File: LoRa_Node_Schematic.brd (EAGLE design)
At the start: 51 x 23 mm, 52 parts, among them J1 ZX62D-B-5PA8, J3 B2B-PH-K-S(LF)(SN), U1 ATSAMD21G18A-AU, U2 RFM95W-868S2SMALL, U3 AP2112K-3.3, U4 MCP73831-2ACI/OT, U5 SHT40-AD1B-R2, Y1 32.768KHZ

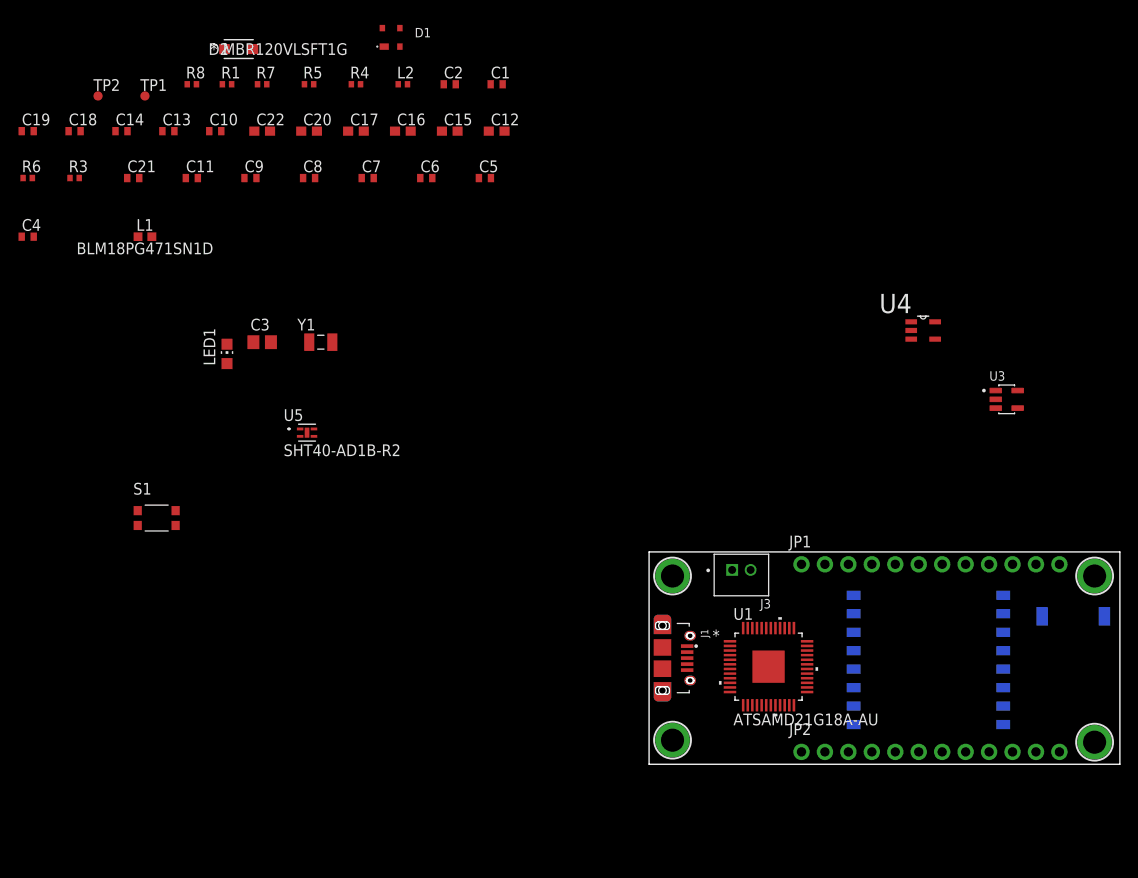
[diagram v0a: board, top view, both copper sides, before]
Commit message: update
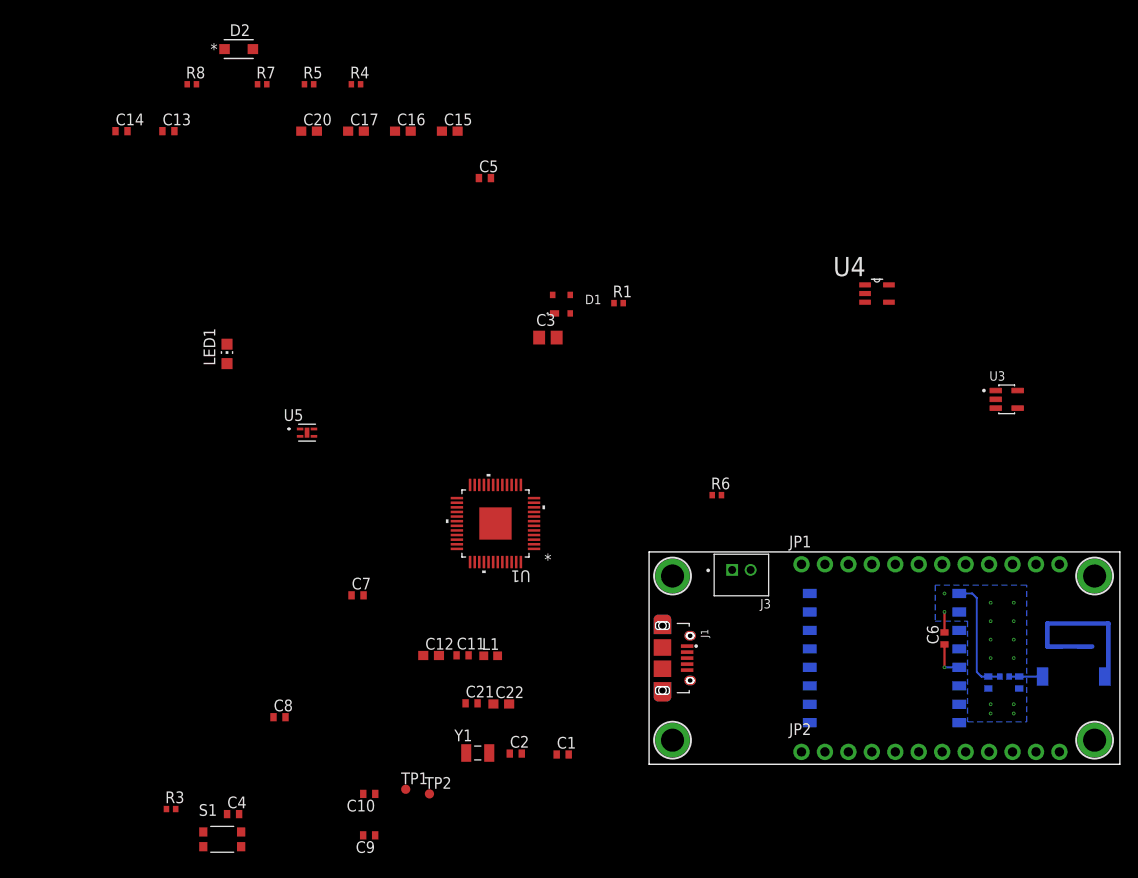
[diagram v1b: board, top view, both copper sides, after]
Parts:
- moved C19 122.9 mm to (40.1, 8.85), flipped to the bottom, turned to 270 degrees
- moved C18 115.6 mm to (36.8, 8.85), flipped to the bottom, turned to 270 degrees
- moved L2 91.5 mm to (38.5, 9.50), flipped to the bottom, turned to 180 degrees
- moved TP2 83.7 mm to (-23.8, -3.21)
- moved R6 82.2 mm to (7.34, 29.1)
- moved TP1 80.2 mm to (-26.4, -2.71)
- moved C6 75.1 mm to (32.0, 13.6), turned to 90 degrees
- moved C10 73.7 mm to (-30.3, -3.21), turned to 180 degrees
- moved C1 73.0 mm to (-9.36, 1.06)
- moved C2 72.9 mm to (-14.4, 1.16)
- moved C9 72.4 mm to (-30.3, -7.70), turned to 180 degrees
- moved R3 69.1 mm to (-51.8, -4.85)
- moved C21 67.7 mm to (-19.2, 6.60)
- moved C22 67.2 mm to (-16.0, 6.53)
- moved C4 66.4 mm to (-45.1, -5.40)
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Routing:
- net ANTENNA: track 0.00 -> 12.8 mm
- net +3V3: track 0.00 -> 4.08 mm, vias 0 -> 1
- net ANTENNA_L: track 0.00 -> 3.88 mm
- net GND: track 0.00 -> 2.22 mm, vias 0 -> 14
- added copper zone on layer 16, net GND
- added copper zone on layer 3, net GND

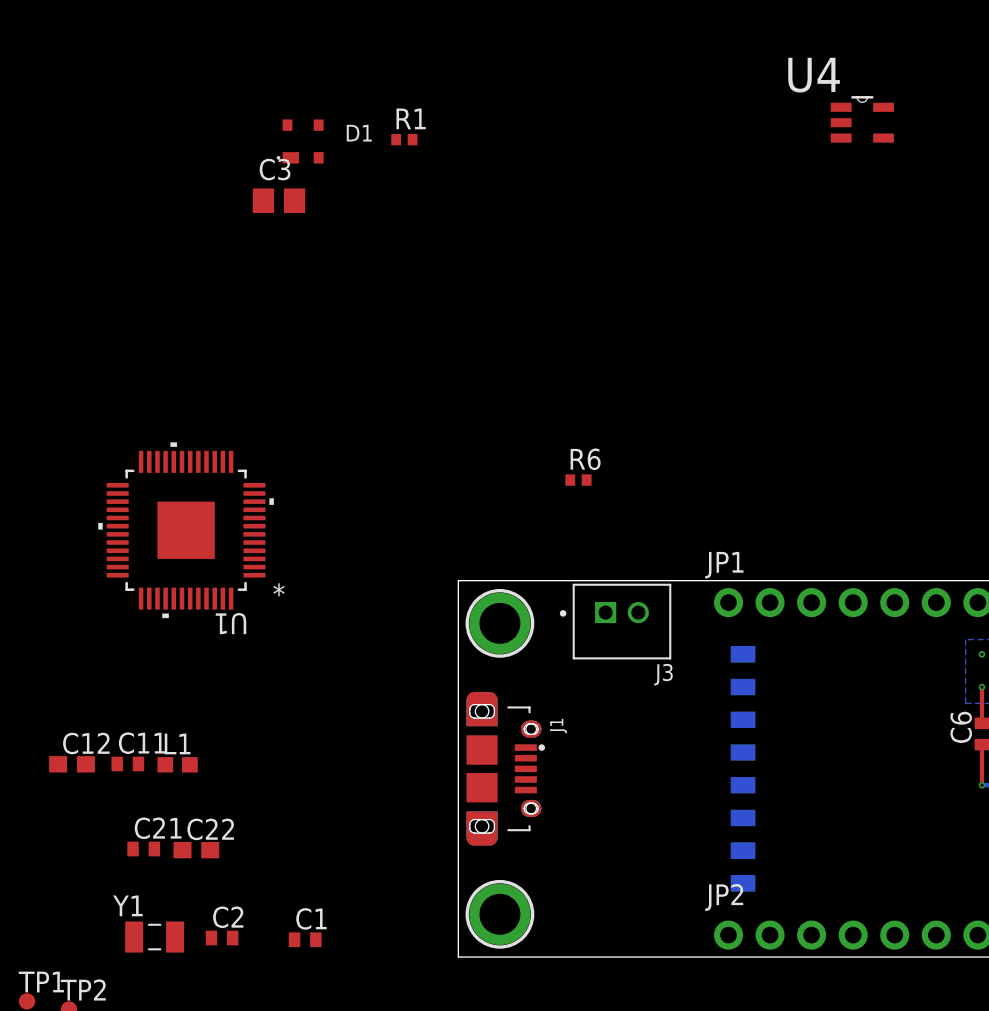
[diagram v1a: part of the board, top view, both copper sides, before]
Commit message: update
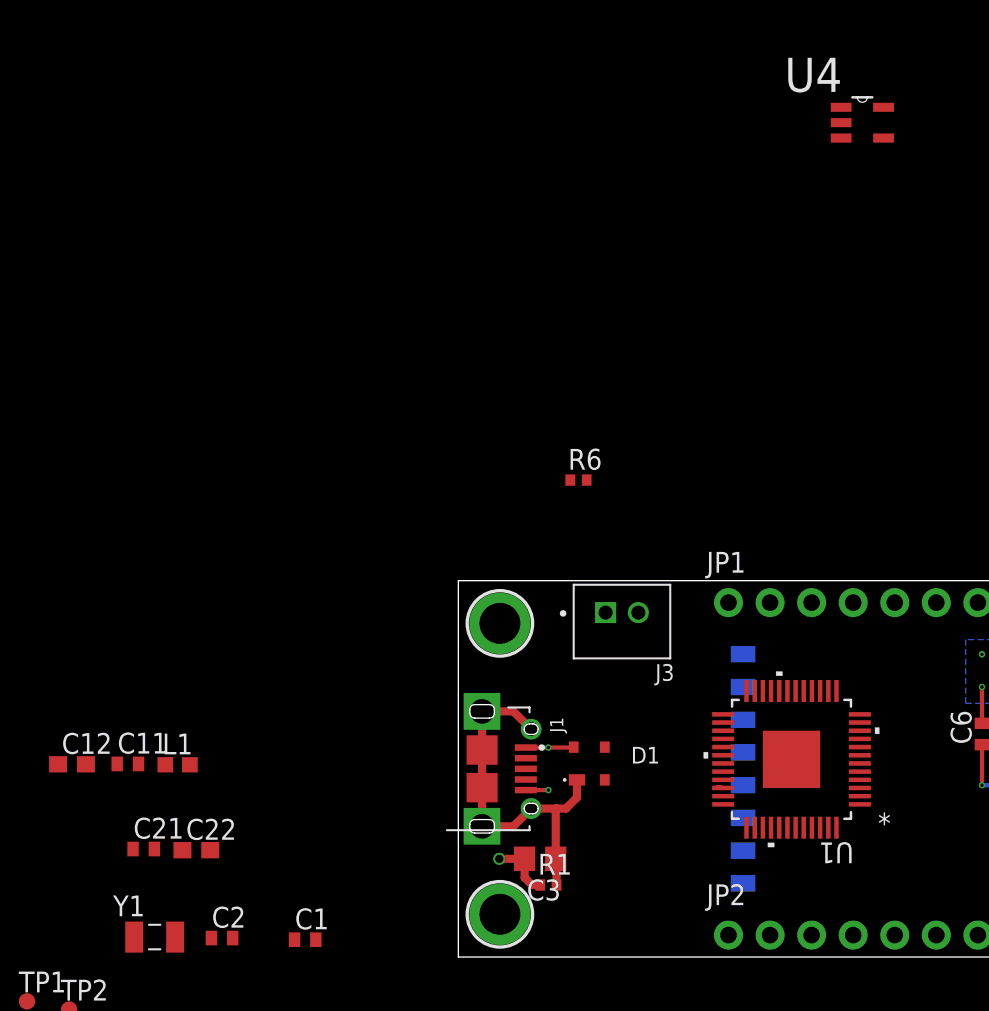
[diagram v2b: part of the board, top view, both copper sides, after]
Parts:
- moved R1 46.4 mm to (5.50, 4.40)
- moved C3 43.3 mm to (5.00, 6.00), turned to 180 degrees
- moved D1 41.8 mm to (8.00, 11.8)
- moved U1 39.6 mm to (20.4, 12.1)
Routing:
- net USB_SHIELD: track 0.00 -> 23.9 mm
- net GND: track 2.22 -> 7.43 mm, vias 14 -> 16
- net VBUS: track 0.00 -> 2.94 mm, vias 0 -> 1

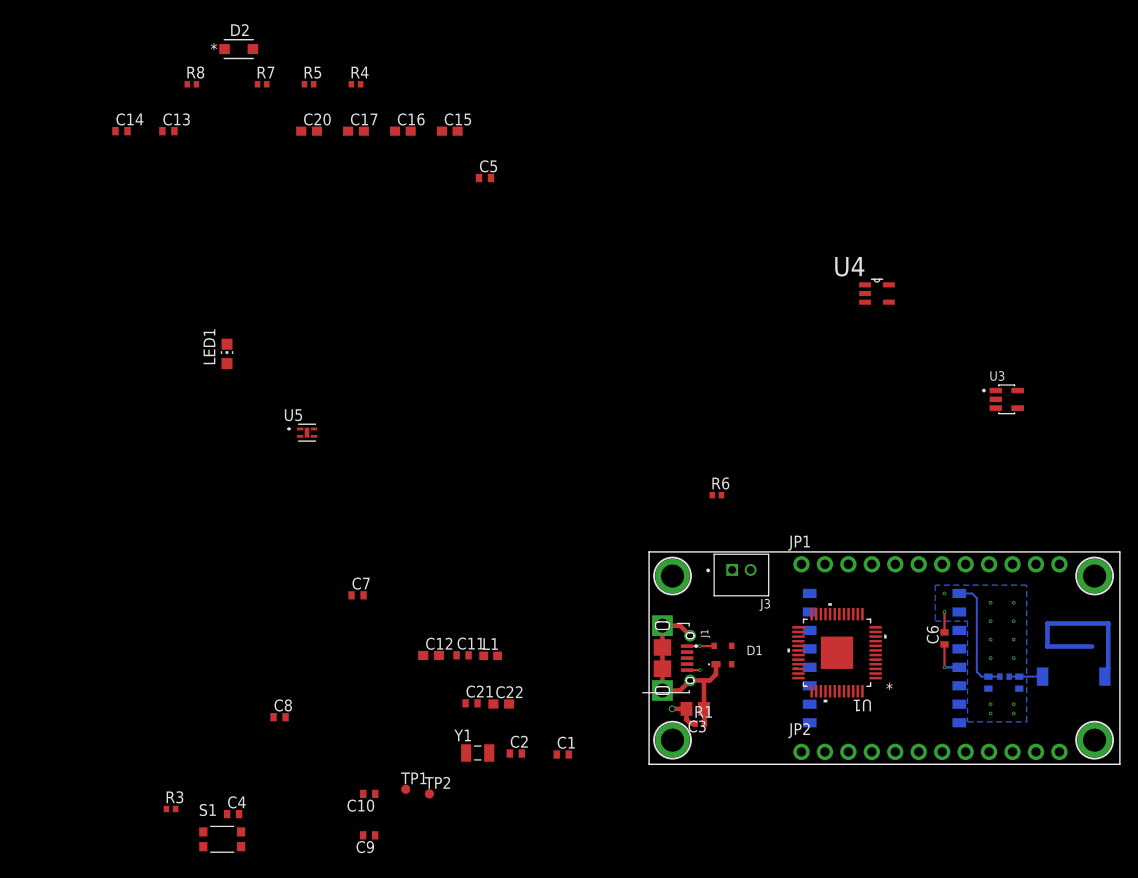
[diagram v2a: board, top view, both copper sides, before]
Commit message: update
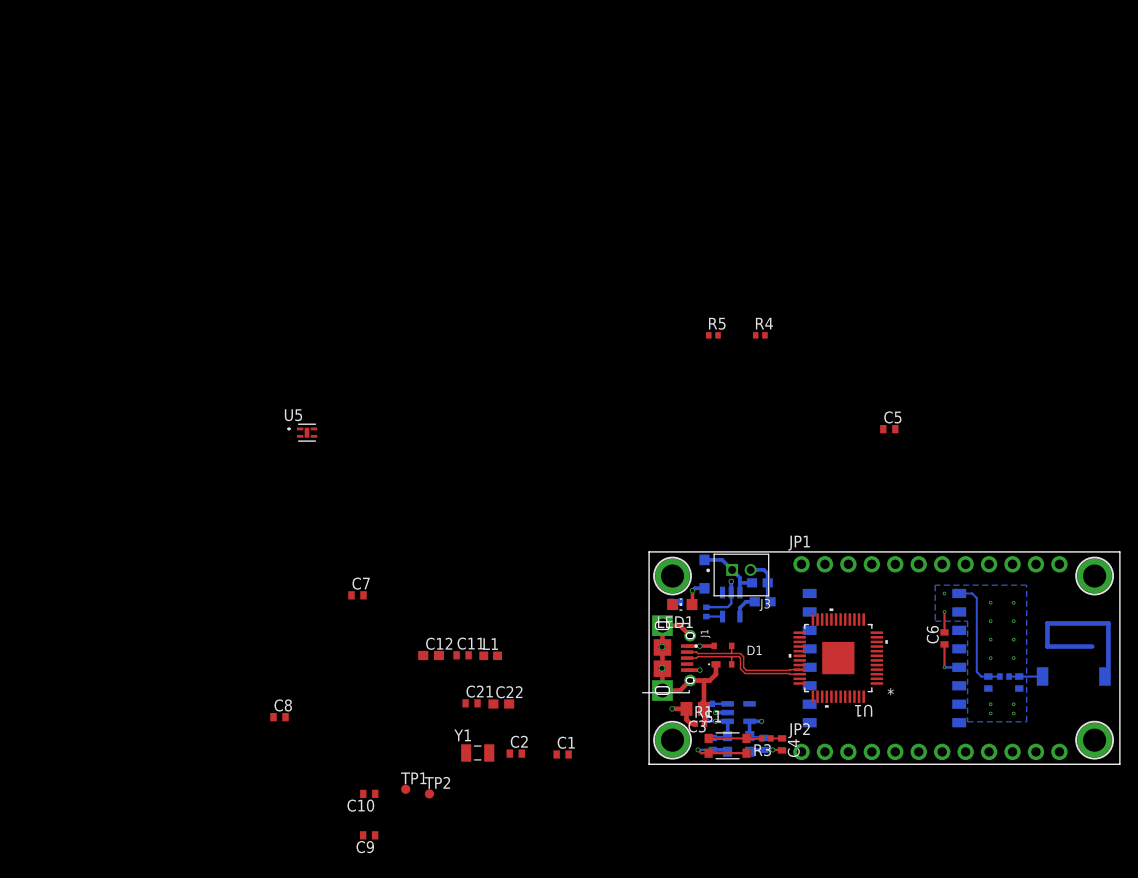
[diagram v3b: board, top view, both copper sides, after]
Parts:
- moved C14 96.2 mm to (12.5, 2.20), flipped to the bottom, turned to 270 degrees
- moved C13 88.8 mm to (6.90, 2.20), flipped to the bottom, turned to 270 degrees
- moved C20 81.8 mm to (10.9, 2.20), flipped to the bottom, turned to 270 degrees
- moved R8 76.8 mm to (2.90, 17.6), flipped to the bottom, turned to 180 degrees
- moved D2 76.0 mm to (6.00, 20.6), flipped to the bottom, turned to 90 degrees
- moved R7 74.7 mm to (6.20, 16.5), flipped to the bottom, turned to 90 degrees
- moved C15 72.9 mm to (8.50, 2.20), flipped to the bottom, turned to 270 degrees
- moved C17 67.4 mm to (12.3, 17.6), flipped to the bottom, turned to 180 degrees
- moved R3 64.9 mm to (12.7, 2.80), turned to 180 degrees
- moved C16 62.4 mm to (12.0, 19.6), flipped to the bottom, turned to 180 degrees
- moved C4 59.9 mm to (14.4, 2.15), turned to 270 degrees
- moved LED1 56.3 mm to (3.60, 17.3), turned to 90 degrees
- moved S1 55.7 mm to (8.50, 2.00)
- moved C5 51.6 mm to (26.0, 36.3)
- moved R4 51.6 mm to (12.1, 46.5)
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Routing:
- net GND: track 7.43 -> 31.5 mm, vias 16 -> 20
- net USB_D_N: track 0.00 -> 14.6 mm
- net USB_D_P: track 0.26 -> 14.6 mm
- net VBUS: track 2.94 -> 16.1 mm, vias 1 -> 3
- net VBAT: track 0.00 -> 7.56 mm
- net RESETN_R: track 0.00 -> 5.75 mm
- net +3V3: track 4.08 -> 8.68 mm, vias 1 -> 2
- net VBAT_PROG: track 0.00 -> 1.76 mm
- net 3V3_EN: track 0.00 -> 1.67 mm
- net RESETN: track 0.00 -> 1.20 mm
- net USB_SHIELD: vias 0 -> 2

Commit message: update
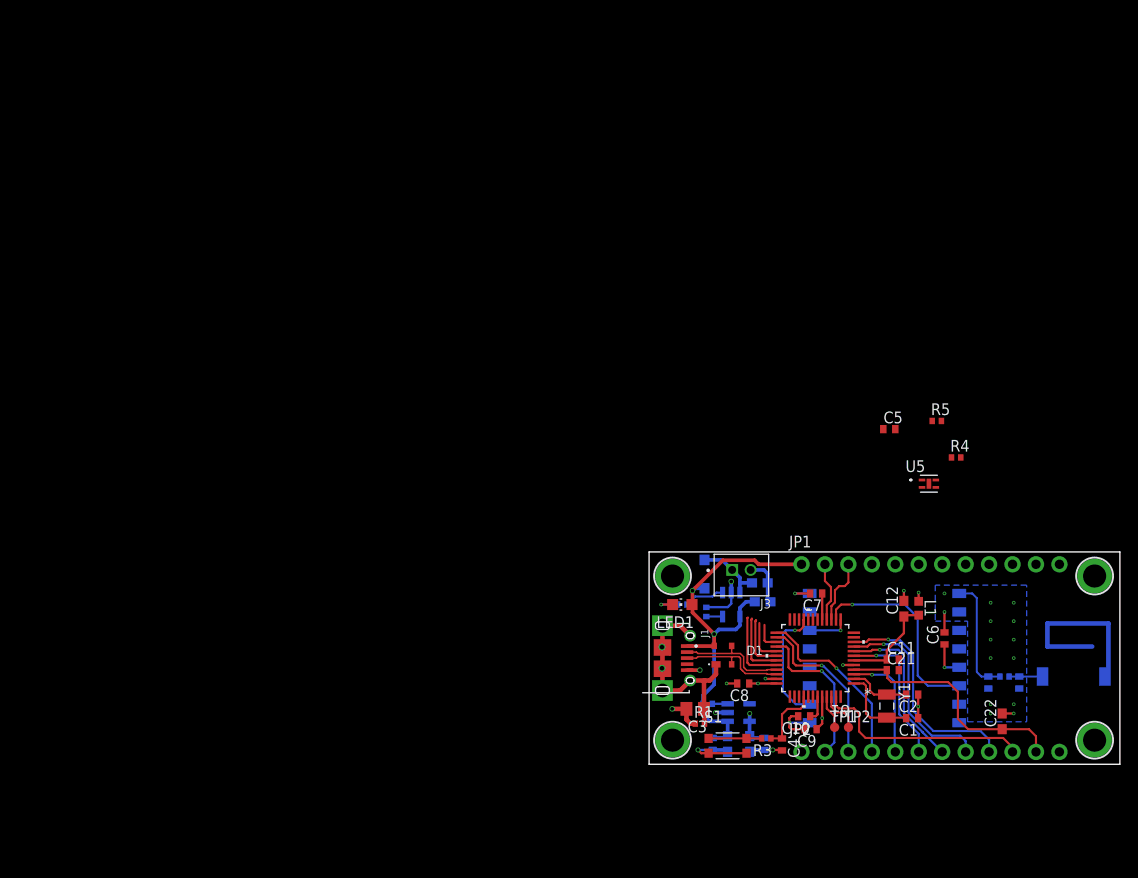
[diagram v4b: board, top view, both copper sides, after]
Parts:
- moved U5 67.6 mm to (30.3, 30.4)
- moved C22 54.3 mm to (38.2, 4.65), turned to 90 degrees
- moved C12 51.5 mm to (27.6, 16.9), turned to 90 degrees
- moved C8 50.4 mm to (10.2, 8.75), turned to 180 degrees
- moved C7 49.7 mm to (18.1, 18.5), turned to 180 degrees
- moved C9 49.2 mm to (17.5, 3.80)
- moved C10 47.9 mm to (16.8, 5.20)
- moved TP1 46.9 mm to (20.1, 4.00)
- moved L1 46.6 mm to (29.2, 16.9), turned to 270 degrees
- moved C11 46.6 mm to (26.4, 11.3)
- moved TP2 46.0 mm to (21.6, 4.00)
- moved C21 45.8 mm to (26.4, 10.2)
- moved Y1 44.6 mm to (25.8, 6.30), turned to 270 degrees
- moved C2 43.4 mm to (28.5, 7.55), turned to 180 degrees
- moved C1 38.1 mm to (28.5, 5.00), turned to 180 degrees
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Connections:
- net A0: now also JP2.5; no longer JP2.2
- net A1: now also JP2.6; no longer JP2.3
- net A2: now also JP2.7; no longer JP2.4
- net A3: now also JP2.8; no longer JP2.5
- net A4: now also JP2.9; no longer JP2.6
- net A5: now also JP2.10; no longer JP2.7
- net AREF: now also JP2.11; no longer JP2.8
- net GND: no longer U1.EPAD
- net SPI_MISO: now also JP2.2; no longer JP2.11
- net SPI_MOSI: now also JP2.4; no longer JP2.10
- net SPI_SCK: now also JP2.3; no longer JP2.9
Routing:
- net VBUS: track 16.1 -> 47.2 mm, vias 3 -> 2
- net AREF: track 0.00 -> 26.6 mm
- net A4: track 0.00 -> 24.2 mm, vias 0 -> 1
- net A5: track 0.00 -> 23.6 mm
- net IRQ_LORA: track 0.00 -> 22.0 mm, vias 0 -> 1
- net A3: track 0.00 -> 21.4 mm, vias 0 -> 1
- net SPI_MOSI: track 0.00 -> 19.5 mm, vias 0 -> 1
- net A2: track 0.00 -> 17.9 mm, vias 0 -> 1
- net SPI_SCK: track 0.00 -> 17.8 mm, vias 0 -> 1
- net GND: track 31.5 -> 49.2 mm, vias 20 -> 27
- net SPI_MISO: track 0.00 -> 16.9 mm, vias 0 -> 1
- net A1: track 0.00 -> 16.1 mm, vias 0 -> 1
- net MISO_LORA: track 0.00 -> 13.1 mm, vias 0 -> 1
- net A0: track 0.00 -> 12.4 mm, vias 0 -> 1
- net VDDANA: track 0.00 -> 10.7 mm
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- added copper zone on layer 2, net +3V3
